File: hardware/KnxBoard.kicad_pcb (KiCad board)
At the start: 4 copper layers, 40 parts, among them J1 Conn_01x10, J2 Conn_01x12, J3 Conn_01x12, J4 Conn_01x02_Male, U1 NCN5130, U2 STM32L432KCUx, X1 FA-238

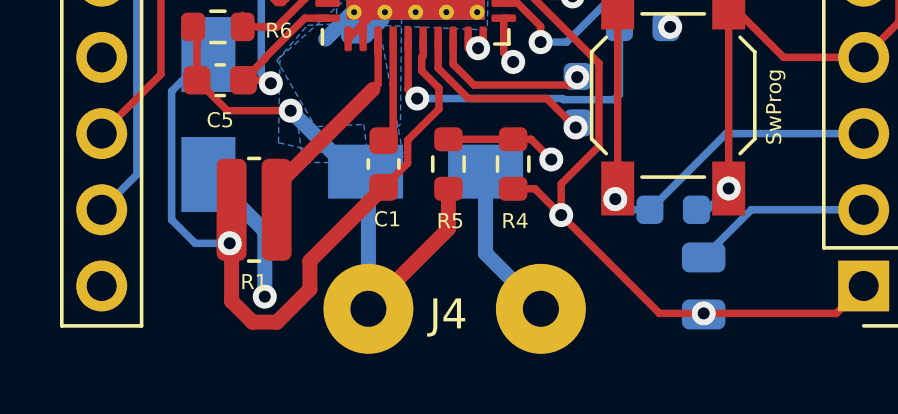
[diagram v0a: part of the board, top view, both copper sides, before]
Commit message: Add text
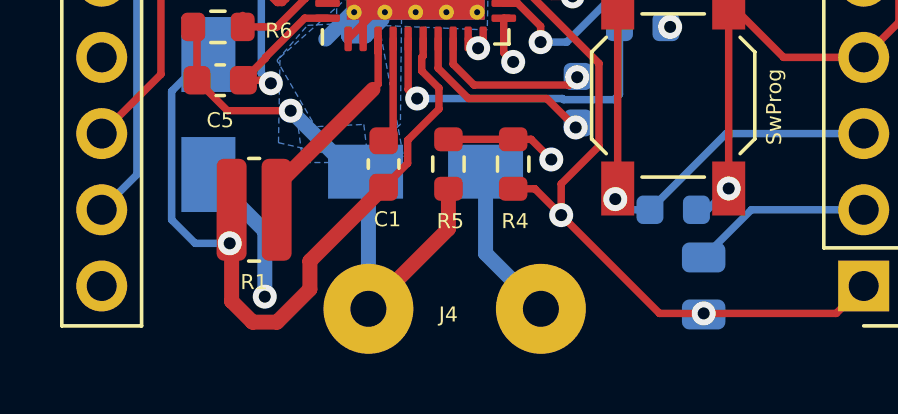
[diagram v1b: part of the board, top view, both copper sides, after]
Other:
- board text added: "CLK16"
- board text added: "PA1"
- board text added: "PC14"
- board text added: "PC15"
- board text added: "UART_TX"
